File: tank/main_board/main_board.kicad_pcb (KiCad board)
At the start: 2 copper layers, 66.5 x 56.2 mm, 43 parts, among them J1 PowerOut, J10 PowerMotor, J11 SigOut, J12 Spk, J13 LEDs, J14 M1, J15 M2, J16 M0, J2 PowerIn, J3 Encoder0, J4 Encoder1, J5 Encoder2, J6 Encoder3, J7 Bump0, J8 Bump1, J9 Programming Header, Q1 2N3904, U1 L7805, U2 ATMEGA328P-PU, U3 SN74HC595, U4 TB6612FNG, U5 TB6612FNG, Y1 Crystal

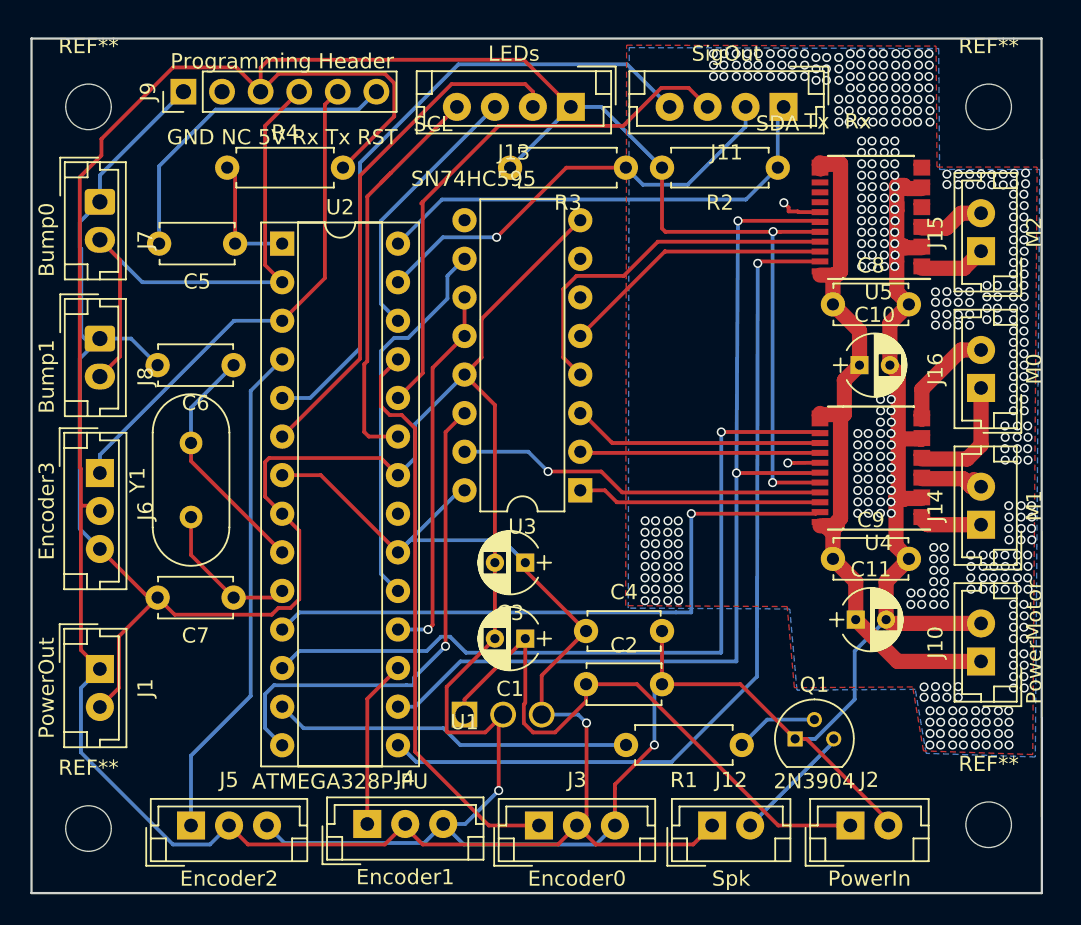
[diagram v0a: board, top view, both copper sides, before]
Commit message: l293d version
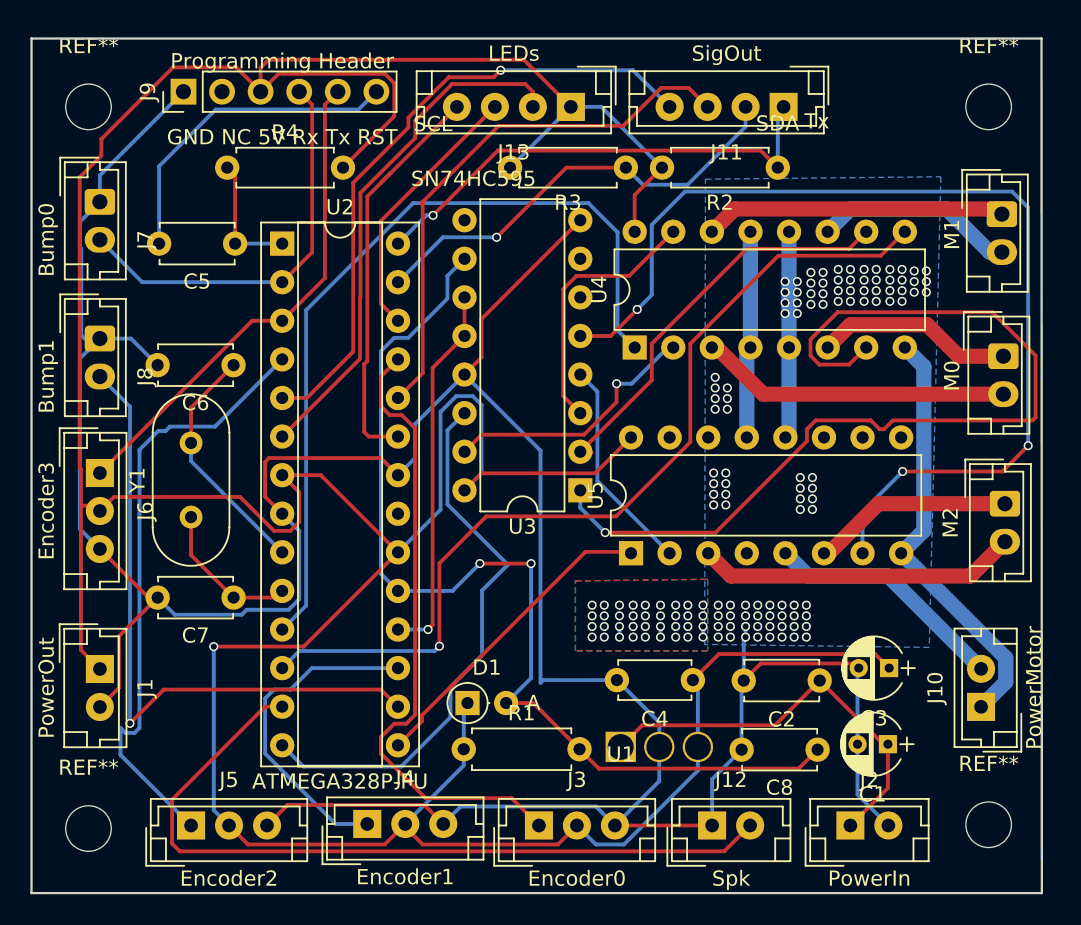
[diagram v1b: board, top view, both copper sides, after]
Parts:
- removed C10, C11: CP, Capacitors_THT:CP_Radial_D4.0mm_P2.00mm
- removed C9: C, Capacitor_THT:C_Disc_D4.7mm_W2.5mm_P5.00mm
- removed J14: M1, JST:JST_EH_B02B-EH-A_02x2.50mm_Straight
- removed J15: M2, JST:JST_EH_B02B-EH-A_02x2.50mm_Straight
- removed J16: M0, JST:JST_EH_B02B-EH-A_02x2.50mm_Straight
- removed Q1: 2N3904, TO_SOT_Packages_THT:TO-92_Molded_Narrow
- added D1: D, Diode_THT:D_DO-35_SOD27_P2.54mm_Vertical_AnodeUp, F.Cu at (126.2, 117.2)
- added M0: M0, Connector_JST:JST_EH_B2B-EH-A_1x02_P2.50mm_Vertical, F.Cu at (161.5, 94.4)
- added M1: M1, Connector_JST:JST_EH_B2B-EH-A_1x02_P2.50mm_Vertical, F.Cu at (161.4, 85.1)
- added M2: M2, Connector_JST:JST_EH_B2B-EH-A_1x02_P2.50mm_Vertical, F.Cu at (161.6, 104.1)
- C8: value C -> C_Small
- R1: value R11 -> R; footprint Resistors_THT:R_Axial_DIN0207_L6.3mm_D2.5mm_P7.62mm_Horizontal -> Resistor_THT:R_Axial_DIN0207_L6.3mm_D2.5mm_P7.62mm_Horizontal
- U4, U5: value TB6612FNG -> L293D; footprint Custom:TB6612FNG -> Package_DIP:DIP-16_W7.62mm
- moved C8 29.3 mm to (149.2, 120.3), turned to 180 degrees
- moved U5 27.5 mm to (137.0, 107.4), turned to 90 degrees
- moved C3 24.9 mm to (153.9, 114.9)
- moved C1 24.9 mm to (153.9, 120.0)
- moved R1 18.3 mm to (126.0, 120.3), turned to 0 degrees
- moved U4 17.9 mm to (137.2, 93.8), turned to 90 degrees
- moved C2 15.4 mm to (149.4, 115.8), turned to 180 degrees
- moved U1 10.5 mm to (136.3, 120.1)
- moved C4 7.74 mm to (141.0, 115.7), turned to 180 degrees
- moved J10 2.99 mm to (160.0, 117.5)
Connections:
- C8 pad 1: Vm -> SRCLR
- J12 pad 1: 4.5V -> GND
- J12 pad 2: Net-(J12-Pad2) -> SPK
- J7 pad 2: Bump -> Bump0
- J8 pad 2: Bump -> Bump1
- J9 pad 4: Bump -> Bump0
- R1 pad 1: Net-(Q1-Pad2) -> 4.5V
- R1 pad 2: SPK -> SRCLR
- U2 pad 16: MEnable -> Bump1
- U2 pad 2: Bump -> Bump0
- U4 pad 1: Net-(J14-Pad1) -> M0PWM
- U4 pad 10: GND -> M1+
- U4 pad 11: Net-(J16-Pad2) -> Net-(J15-Pad2)
- U4 pad 12: Net-(J16-Pad2) -> GND
- U4 pad 13: Vm -> GND
- U4 pad 14: Vm -> Net-(J15-Pad1)
- U4 pad 15: M1PWM -> M1-
- U4 pad 16: M1- -> 4.5V
- U4 pad 2: Net-(J14-Pad1) -> M0+
- U4 pad 3: GND -> Net-(J14-Pad2)
- U4 pad 5: Net-(J14-Pad2) -> GND
- U4 pad 6: Net-(J14-Pad2) -> Net-(J14-Pad1)
- U4 pad 7: Net-(J16-Pad1) -> M0-
- U4 pad 8: Net-(J16-Pad1) -> Vm
- U4 pad 9: GND -> M1PWM
- U5 pad 1: Net-(J15-Pad1) -> M2PWM
- U5 pad 10: GND -> Net-(U5-Pad10)
- U5 pad 12: Net-(U5-Pad11) -> GND
- U5 pad 13: Vm -> GND
- U5 pad 14: Vm -> Net-(U5-Pad14)
- U5 pad 16: Net-(U5-Pad16) -> 4.5V
- U5 pad 2: Net-(J15-Pad1) -> M2+
- U5 pad 3: GND -> Net-(J16-Pad2)
- U5 pad 5: Net-(J15-Pad2) -> GND
- U5 pad 6: Net-(J15-Pad2) -> Net-(J16-Pad1)
- U5 pad 7: Net-(U5-Pad7) -> M2-
- U5 pad 8: Net-(U5-Pad7) -> Vm
- U5 pad 9: GND -> Net-(U5-Pad9)
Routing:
- net MEnable: track 64.0 -> 0.00 mm, vias 2 -> 0
- net M2-: track 18.1 -> 67.8 mm, vias 0 -> 3
- net M0-: track 16.1 -> 62.1 mm, vias 0 -> 1
- net Bump1: track 0.00 -> 43.0 mm, vias 0 -> 1
- net SRCLR: track 25.1 -> 67.4 mm, vias 0 -> 2
- net Bump: track 37.2 -> 0.00 mm
- net M2PWM: track 57.8 -> 20.9 mm, vias 1 -> 0
- net SPK: track 23.7 -> 51.6 mm
- net Bump0: track 0.00 -> 26.9 mm
- net 4.5V: track 240.1 -> 261.1 mm, vias 3 -> 1
- net Vm: track 49.0 -> 28.3 mm
- net Net-(J14-Pad2): track 4.79 -> 20.5 mm
- net Net-(J15-Pad1): track 4.37 -> 19.9 mm
- net Net-(J16-Pad2): track 6.96 -> 21.1 mm
- net 9V: track 40.2 -> 27.5 mm
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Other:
- board text added: "Laser Tag Robot Tank Main Board v0.9 - L293D Edition M.I.A.R. Labs nick.groesz@gmail.com"
- board text removed: "Laser Tag Robot Tank Main Board v0.8 M.I.A.R. Labs nick.groesz@gmail.com"
- board text removed: "Rx"
